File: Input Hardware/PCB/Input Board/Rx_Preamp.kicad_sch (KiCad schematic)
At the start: 44 parts, among them U301 ADA4891, U302 ADA4891

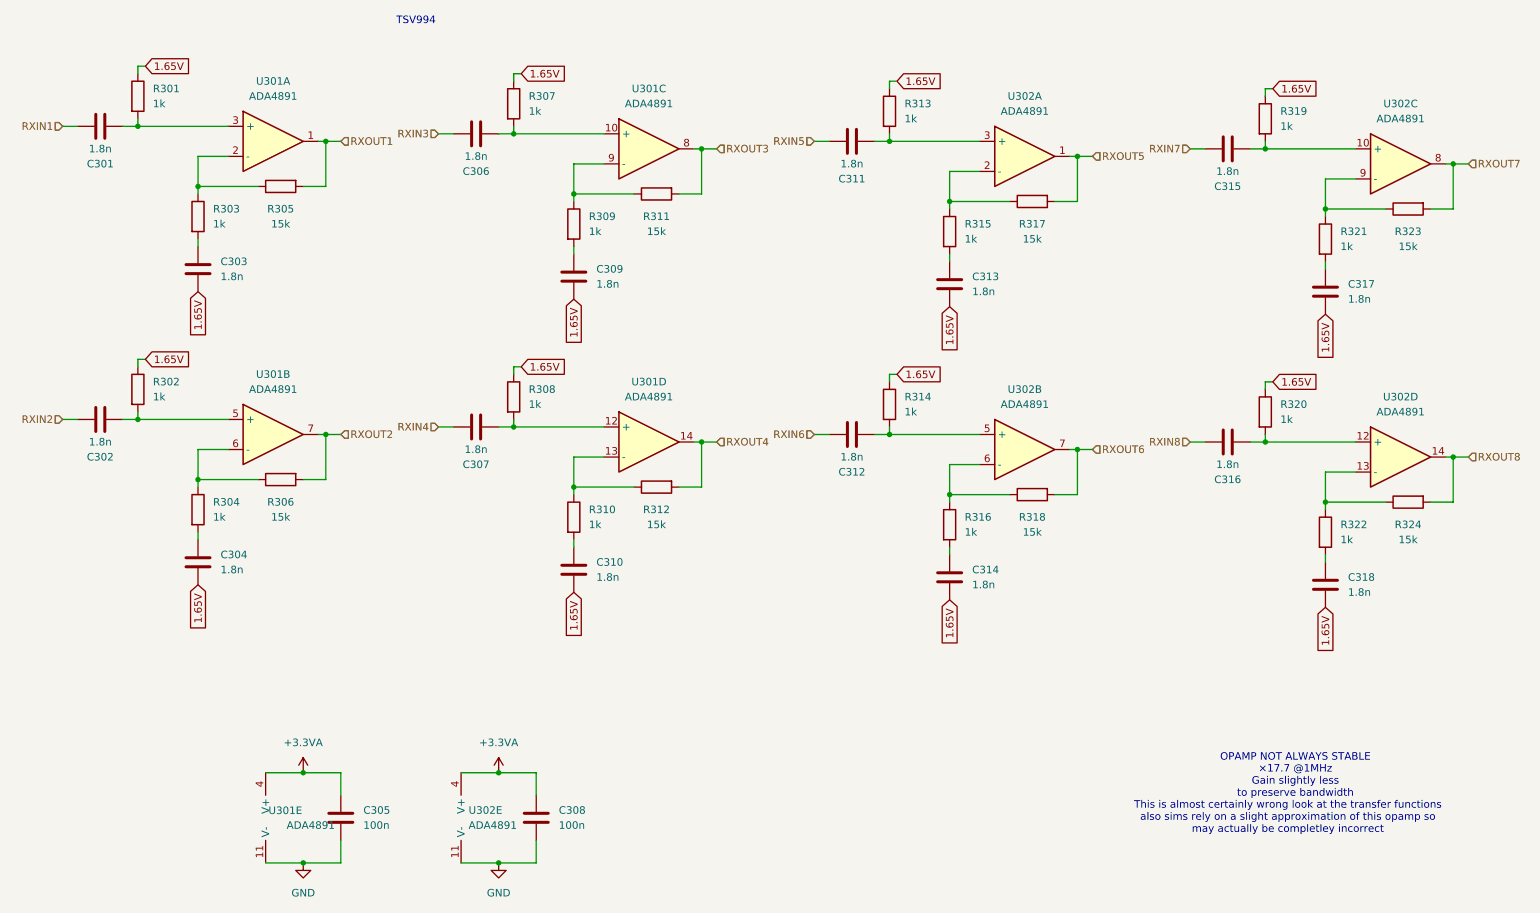
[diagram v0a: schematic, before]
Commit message: opamp part changes
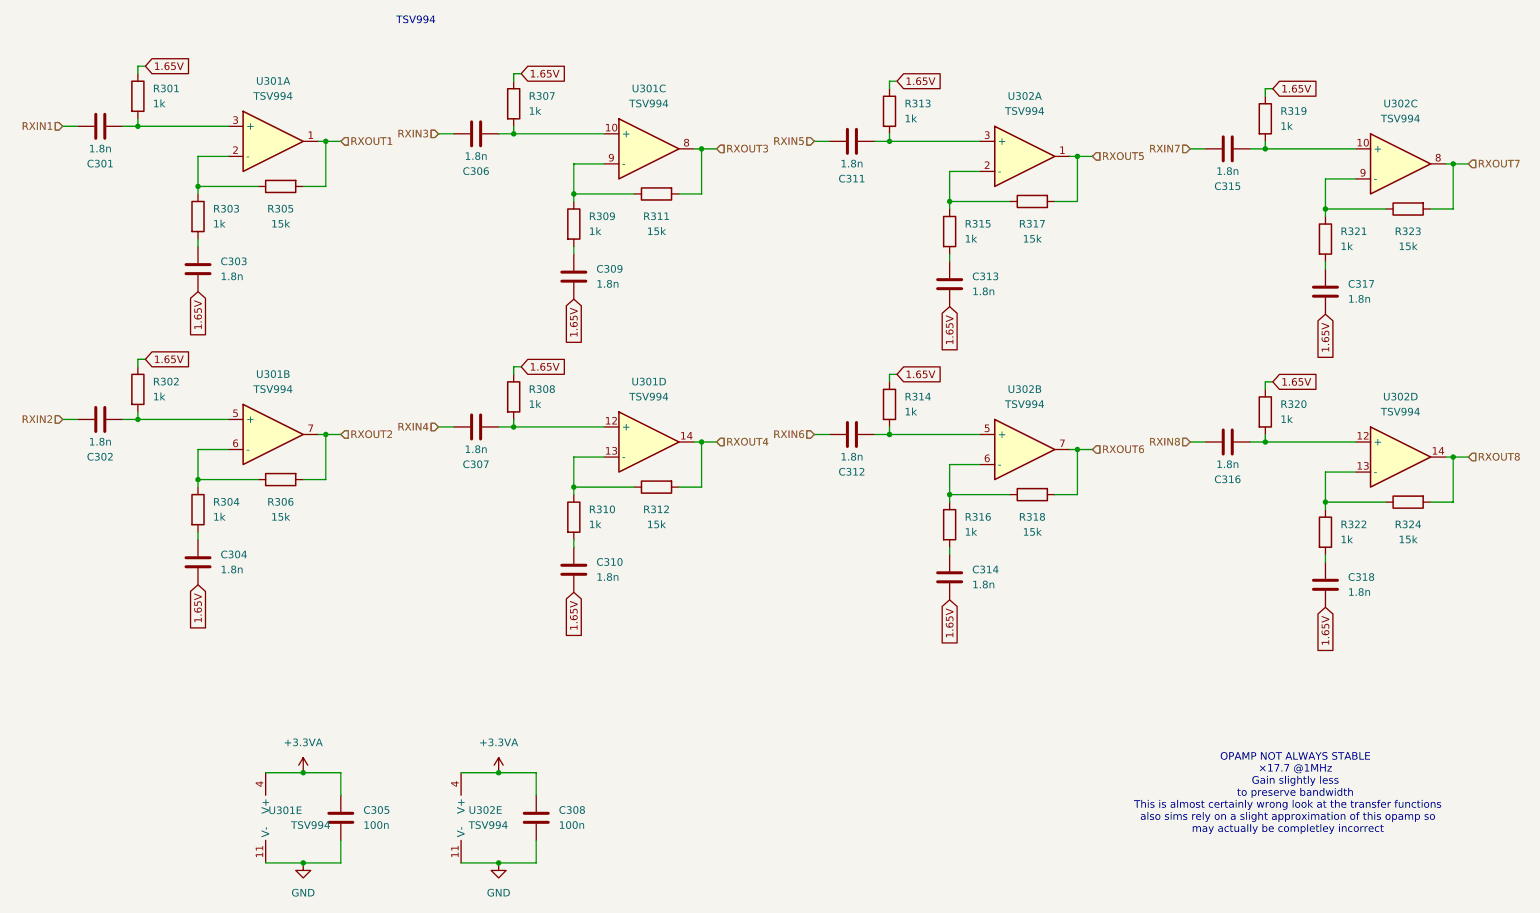
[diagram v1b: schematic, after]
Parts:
- U301, U302: value ADA4891 -> TSV994
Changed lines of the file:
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@@
 			)
 		)
-		(property "Value" "ADA4891"
+		(property "Value" "TSV994"
 			(at 191.77 82.55 0)
 			(effects
@@
 			)
 		)
-		(property "Value" "ADA4891"
+		(property "Value" "TSV994"
 			(at 128.27 31.75 0)
 			(effects
@@
 			)
 		)
-		(property "Value" "ADA4891"
+		(property "Value" "TSV994"
 			(at 64.77 30.48 0)
 			(effects
@@
 			)
 		)
-		(property "Value" "ADA4891"
+		(property "Value" "TSV994"
 			(at 191.77 33.02 0)
 			(effects
@@
 			)
 		)
-		(property "Value" "ADA4891"
+		(property "Value" "TSV994"
 			(at 64.77 80.01 0)
 			(effects
@@
 			)
 		)
-		(property "Value" "ADA4891"
+		(property "Value" "TSV994"
 			(at 97.79 153.6699 0)
 			(effects
@@
 			)
 		)
-		(property "Value" "ADA4891"
+		(property "Value" "TSV994"
 			(at 255.27 83.82 0)
 			(effects
@@
 			)
 		)
-		(property "Value" "ADA4891"
+		(property "Value" "TSV994"
 			(at 255.27 34.29 0)
 			(effects
@@
 			)
 		)
-		(property "Value" "ADA4891"
+		(property "Value" "TSV994"
 			(at 71.12 153.67 0)
 			(effects
@@
 			)
 		)
-		(property "Value" "ADA4891"
+		(property "Value" "TSV994"
 			(at 128.27 81.28 0)
 			(effects

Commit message: Layout Progress
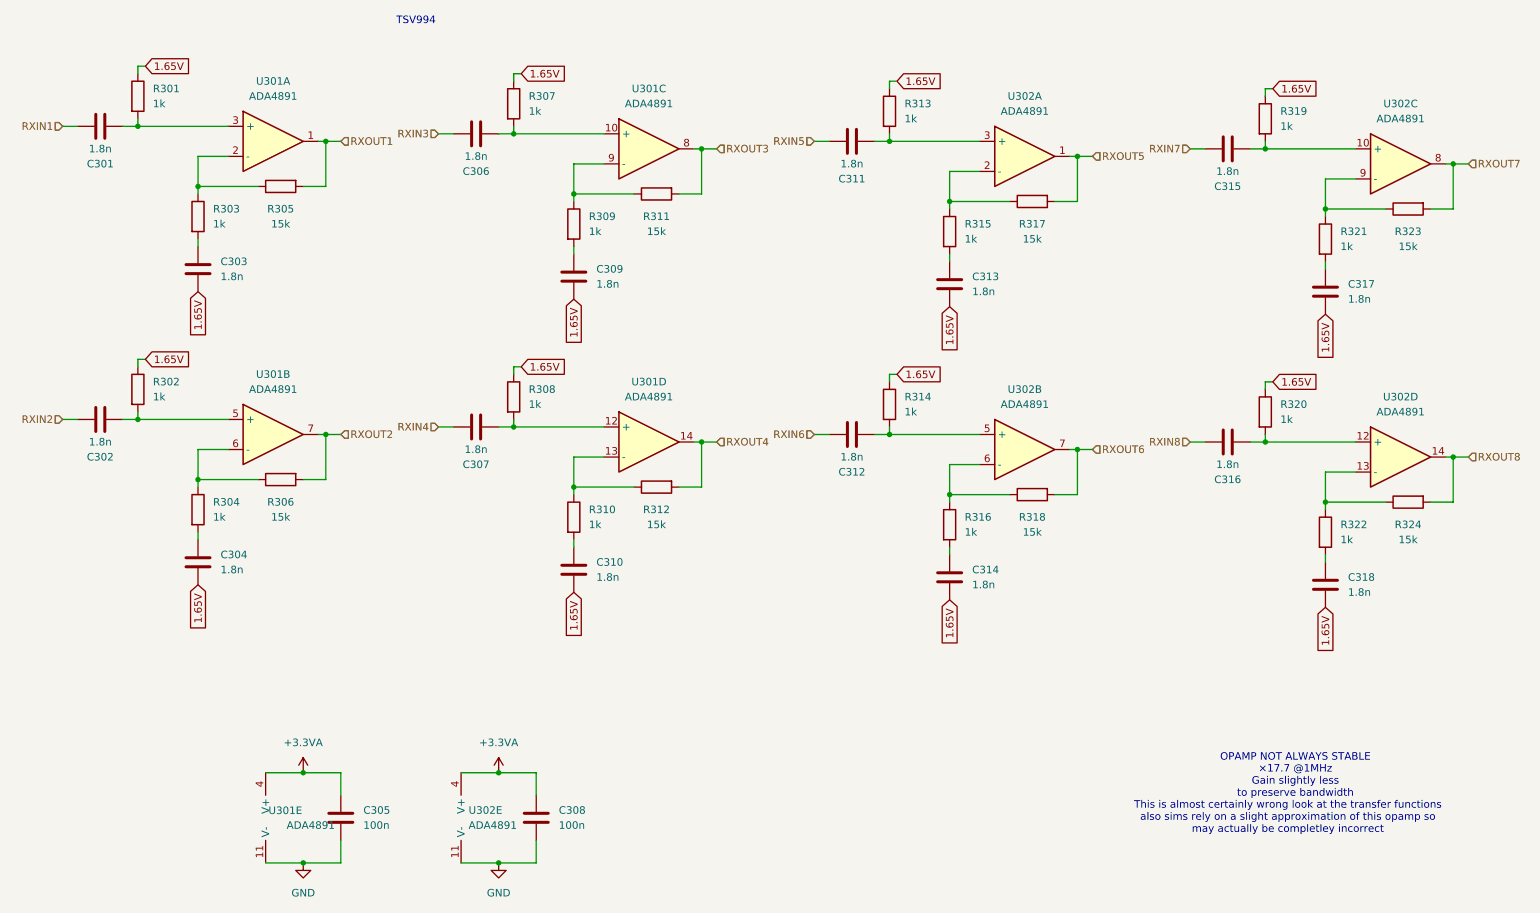
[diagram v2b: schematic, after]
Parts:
- U301, U302: value TSV994 -> ADA4891
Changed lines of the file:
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@@
 			)
 		)
-		(property "Value" "TSV994"
+		(property "Value" "ADA4891"
 			(at 191.77 82.55 0)
 			(effects
@@
 			)
 		)
-		(property "Value" "TSV994"
+		(property "Value" "ADA4891"
 			(at 128.27 31.75 0)
 			(effects
@@
 			)
 		)
-		(property "Value" "TSV994"
+		(property "Value" "ADA4891"
 			(at 64.77 30.48 0)
 			(effects
@@
 			)
 		)
-		(property "Value" "TSV994"
+		(property "Value" "ADA4891"
 			(at 191.77 33.02 0)
 			(effects
@@
 			)
 		)
-		(property "Value" "TSV994"
+		(property "Value" "ADA4891"
 			(at 64.77 80.01 0)
 			(effects
@@
 			)
 		)
-		(property "Value" "TSV994"
+		(property "Value" "ADA4891"
 			(at 97.79 153.6699 0)
 			(effects
@@
 			)
 		)
-		(property "Value" "TSV994"
+		(property "Value" "ADA4891"
 			(at 255.27 83.82 0)
 			(effects
@@
 			)
 		)
-		(property "Value" "TSV994"
+		(property "Value" "ADA4891"
 			(at 255.27 34.29 0)
 			(effects
@@
 			)
 		)
-		(property "Value" "TSV994"
+		(property "Value" "ADA4891"
 			(at 71.12 153.67 0)
 			(effects
@@
 			)
 		)
-		(property "Value" "TSV994"
+		(property "Value" "ADA4891"
 			(at 128.27 81.28 0)
 			(effects
